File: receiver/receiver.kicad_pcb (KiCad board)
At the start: 2 copper layers, 38 x 20 mm, 5 parts, among them J1 LVDS_input, J2 signal_out, U1 SN65LVDT348

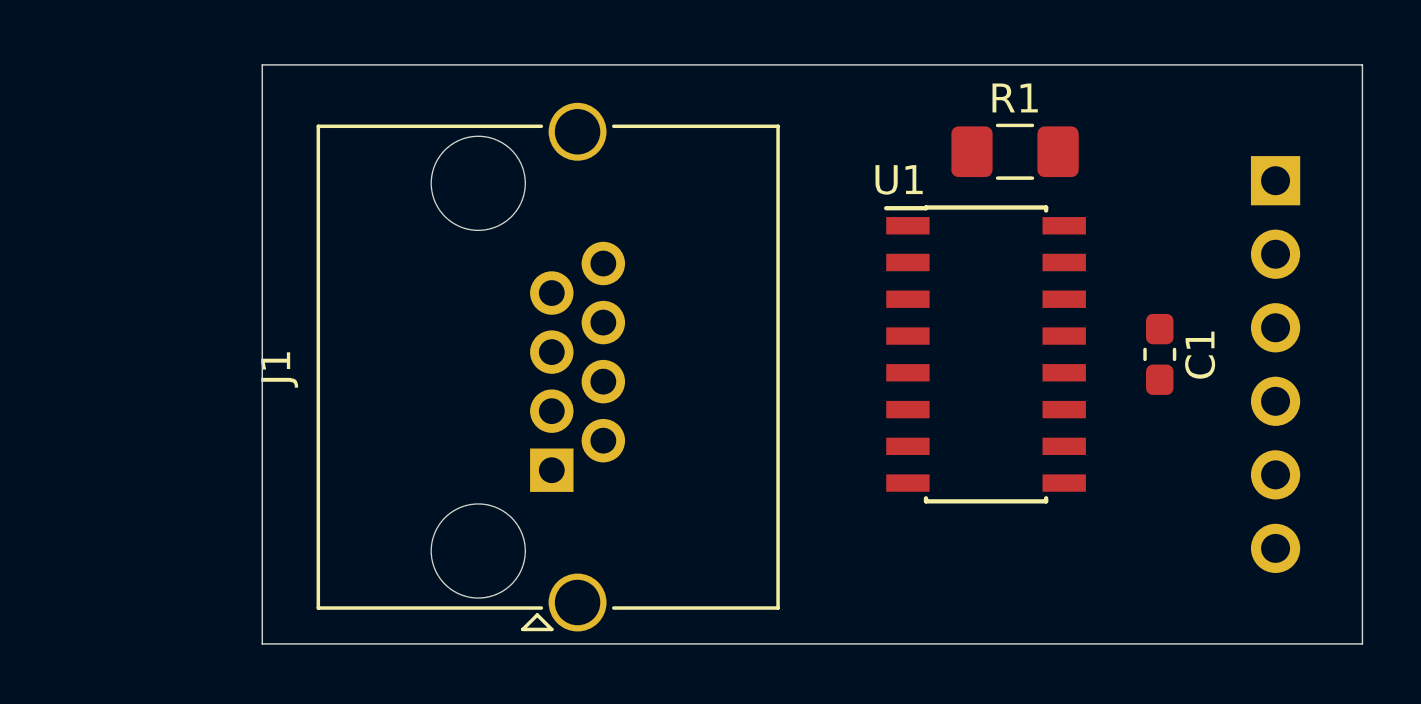
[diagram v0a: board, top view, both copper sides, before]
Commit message: exported..
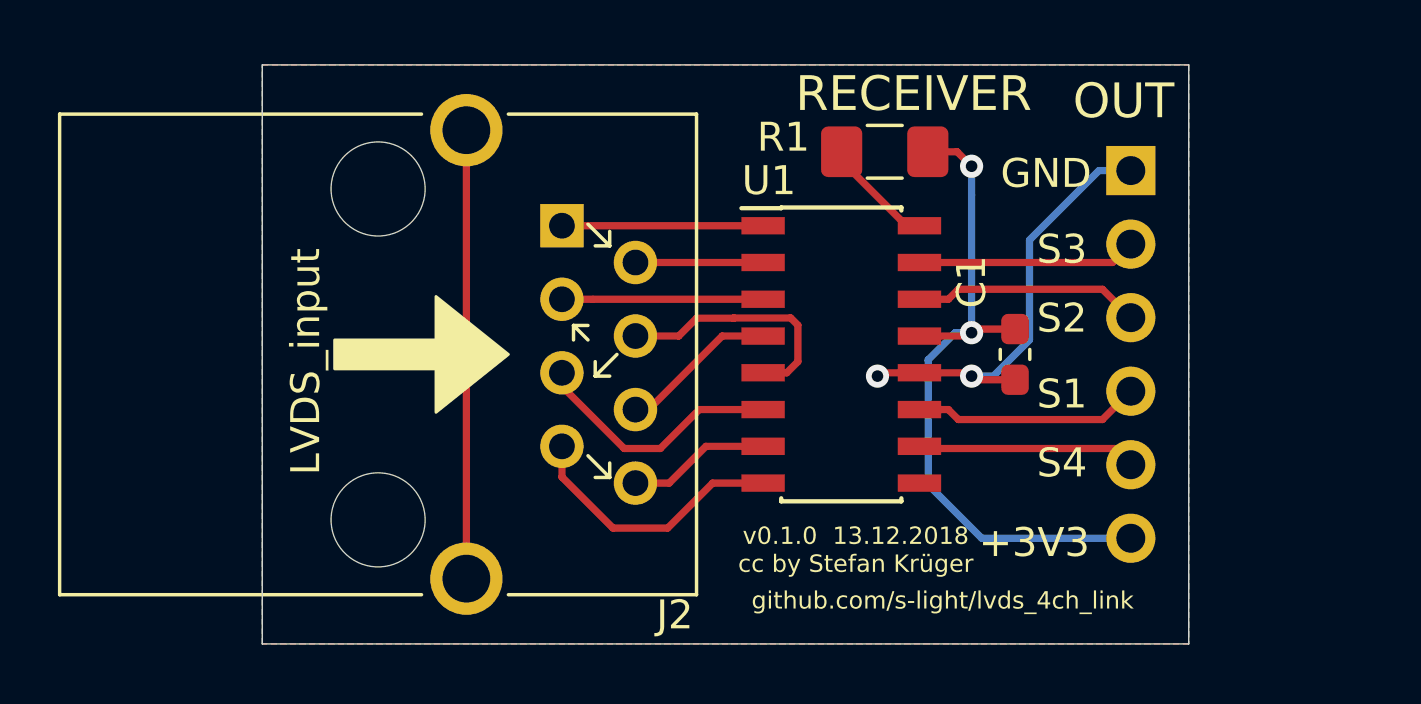
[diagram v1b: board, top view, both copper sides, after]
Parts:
- J1: value LVDS_input -> signal_out; footprint Connector_RJ:RJ45_Amphenol_RJHSE5380 -> Connector_PinHeader_2.54mm:PinHeader_1x06_P2.54mm_Horizontal; moved to B.Cu
- J2: value signal_out -> LVDS_input; footprint Connector_PinHeader_2.54mm:PinHeader_1x06_P2.54mm_Horizontal -> Connector_RJ:RJ45_Stewart_SS-6488S-A-NF; moved to F.Cu
- moved J2 31.6 mm to (54.0, 60.0), turned to 270 degrees
- moved J1 22.5 mm to (80.0, 53.6), turned to 180 degrees
- moved C1 5.00 mm to (76.0, 60.0)
- moved U1 5.00 mm to (70.0, 60.0)
- moved R1 4.50 mm to (71.5, 53.0), turned to 180 degrees
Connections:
- J1 pad 1: /pair3- -> GND
- J1 pad 2: /pair3+ -> /signal3
- J1 pad 3: /pair2+ -> /signal2
- J1 pad 4: /pair1- -> /signal1
- J1 pad 5: /pair1+ -> /signal4
- J1 pad 6: /pair2- -> +3V3
- J2 pad 1: +3V3 -> /pair3-
- J2 pad 2: /signal1 -> /pair3+
- J2 pad 3: /signal2 -> /pair2+
- J2 pad 4: /signal3 -> /pair1-
- J2 pad 5: /signal4 -> /pair1+
- J2 pad 6: GND -> /pair2-
- U1 pad 1: /pair4- -> /pair3-
- U1 pad 10: /signal3 -> /signal4
- U1 pad 11: /signal2 -> /signal1
- U1 pad 14: /signal1 -> /signal2
- U1 pad 15: /signal4 -> /signal3
- U1 pad 2: /pair4+ -> /pair3+
- U1 pad 3: /pair1+ -> /pair2+
- U1 pad 4: /pair1- -> /pair2-
- U1 pad 5: /pair2- -> /pair1-
- U1 pad 6: /pair2+ -> /pair1+
- U1 pad 7: /pair3+ -> /pair4+
- U1 pad 8: /pair3- -> /pair4-
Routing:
- net +3V3: track 0.00 -> 24.8 mm, vias 0 -> 2
- net GND: track 0.00 -> 15.6 mm, vias 0 -> 2
- net Net-(J2-PadSH): track 0.00 -> 15.5 mm
- net /pair4-: track 0.00 -> 9.39 mm
- net /pair1+: track 0.00 -> 8.86 mm
- net /pair1-: track 0.00 -> 8.59 mm
- net /signal2: track 0.00 -> 7.85 mm
- net /signal1: track 0.00 -> 7.85 mm
- net /signal4: track 0.00 -> 7.56 mm
- net /signal3: track 0.00 -> 7.56 mm
- net /pair3-: track 0.00 -> 6.95 mm
- net /pair2+: track 0.00 -> 6.95 mm
- net /pair2-: track 0.00 -> 5.46 mm
- net /pair4+: track 0.00 -> 4.94 mm
- net /pair3+: track 0.00 -> 4.41 mm
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- added copper zone on B.Cu, net GND
- added copper zone on F.Cu, net GND
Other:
- board size 38 x 20 mm -> 32 x 20 mm
- board text added: "+3V3"
- board text added: "GND"
- board text added: "OUT"
- board text added: "RECEIVER"
- board text added: "S1"
- board text added: "S2"
- board text added: "S3"
- board text added: "S4"
- board text added: "github.com/s-light/lvds_4ch_link"
- board text added: "v0.1.0 13.12.2018 cc by Stefan Krüger"
